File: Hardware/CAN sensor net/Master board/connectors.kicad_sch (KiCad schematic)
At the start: 17 parts, among them J1 Micro_SD_Card_Con, J2 USB_B_Micro, J3 Conn_02x05_SWD, J5 532610671, J6 532610671, U2 USBLC6-2SC6

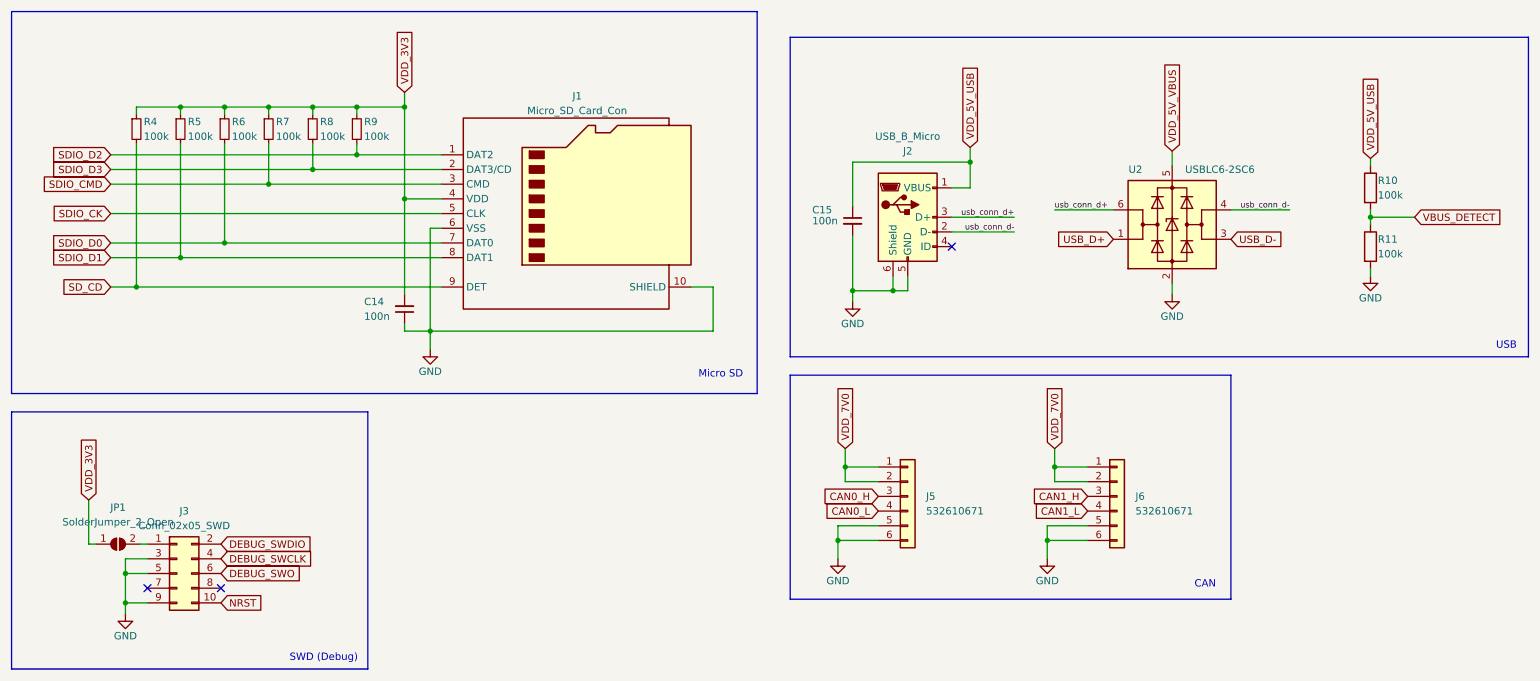
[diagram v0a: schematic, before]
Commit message: Bugfix
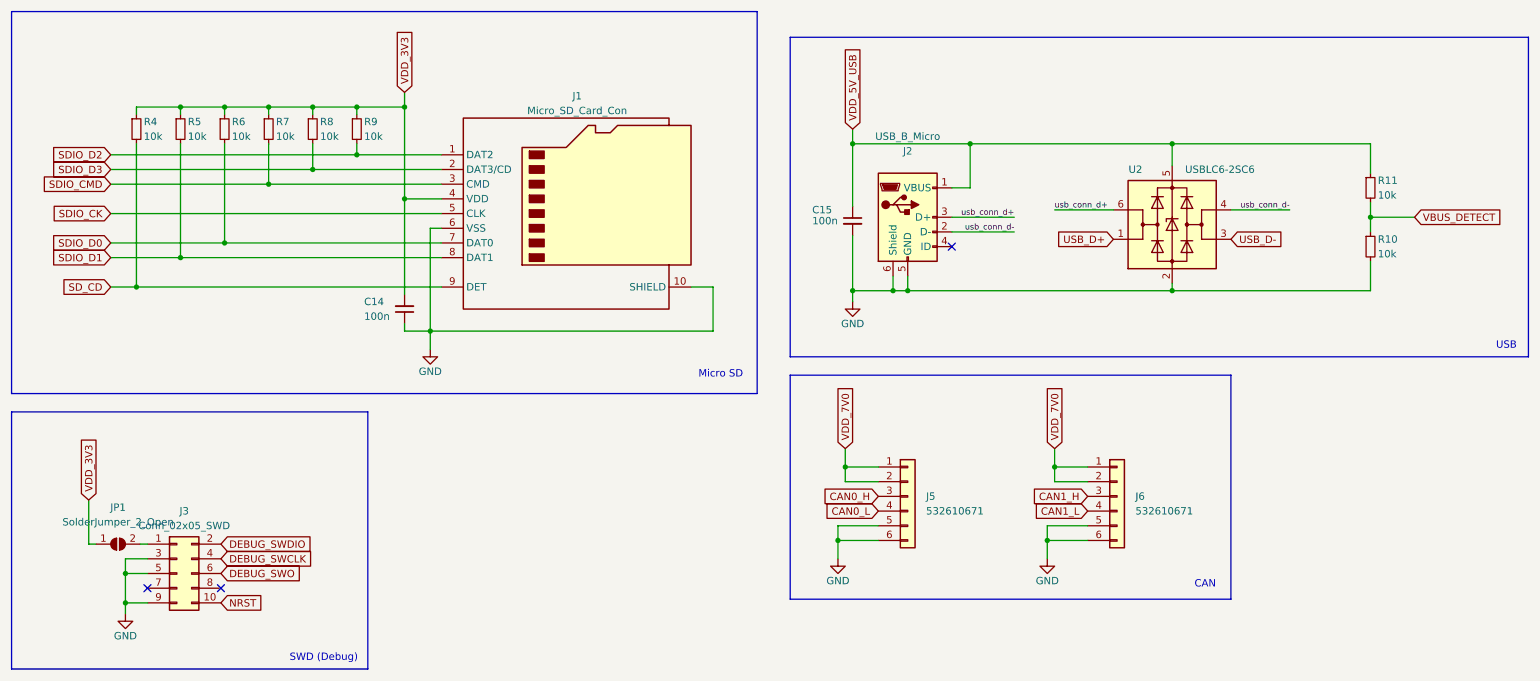
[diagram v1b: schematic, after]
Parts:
- removed R10, R11: 100k, Resistor_SMD:R_0603_1608Metric, symbol Device:R
- added R10, R11: 10k, Resistor_SMD:R_0603_1608Metric, symbol Device:R_Small
- R4, R5, R6, R7, R8, R9: value 100k -> 10k
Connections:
- net VDD_5V_VBUS is gone; now on net VDD_5V_USB: U2.5 (VBUS)
- net GND: now also R10.2
- net VBUS_DETECT: now also R10.1, R11.2
- net VDD_5V_USB: now also R11.1
